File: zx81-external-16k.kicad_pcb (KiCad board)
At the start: 2 copper layers, 59.5 x 39 mm, 10 parts, among them J1 Connector ZX81, U1 CY62256-70PC, U2 74LS00

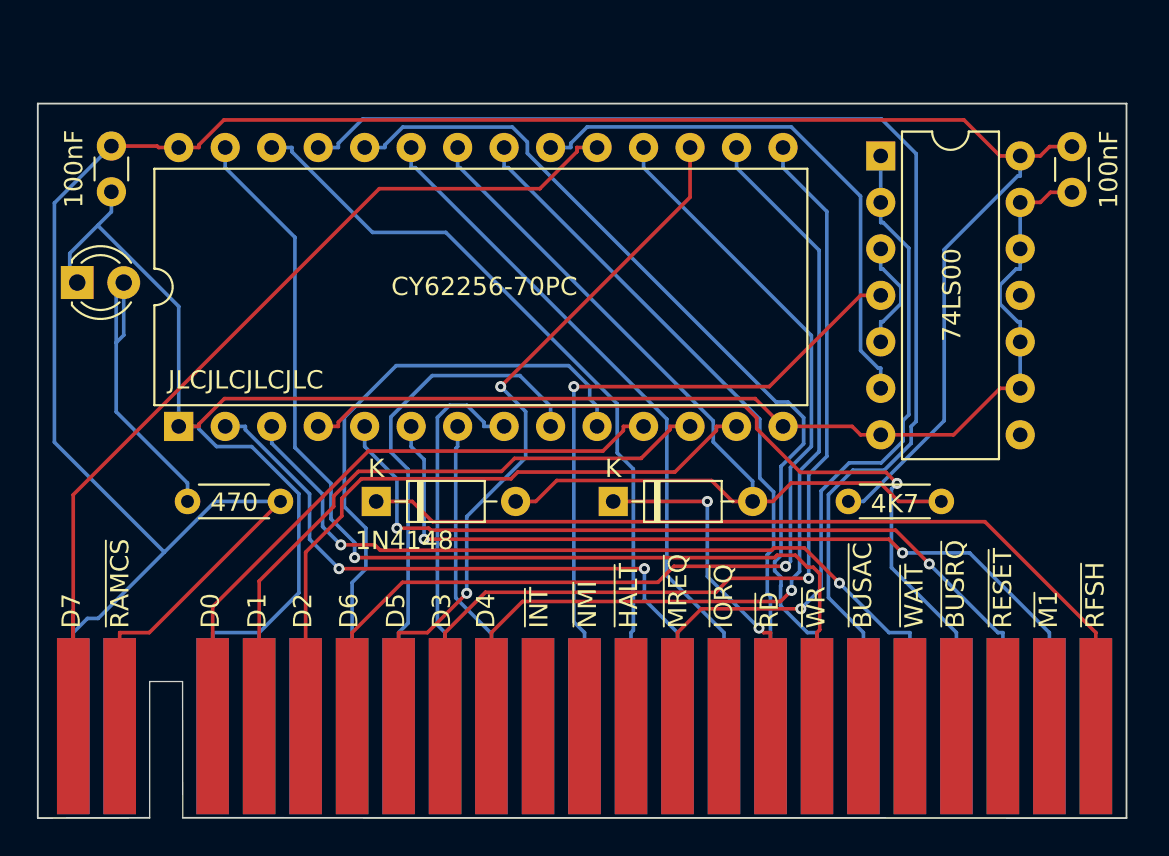
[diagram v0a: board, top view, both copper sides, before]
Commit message: v1.1
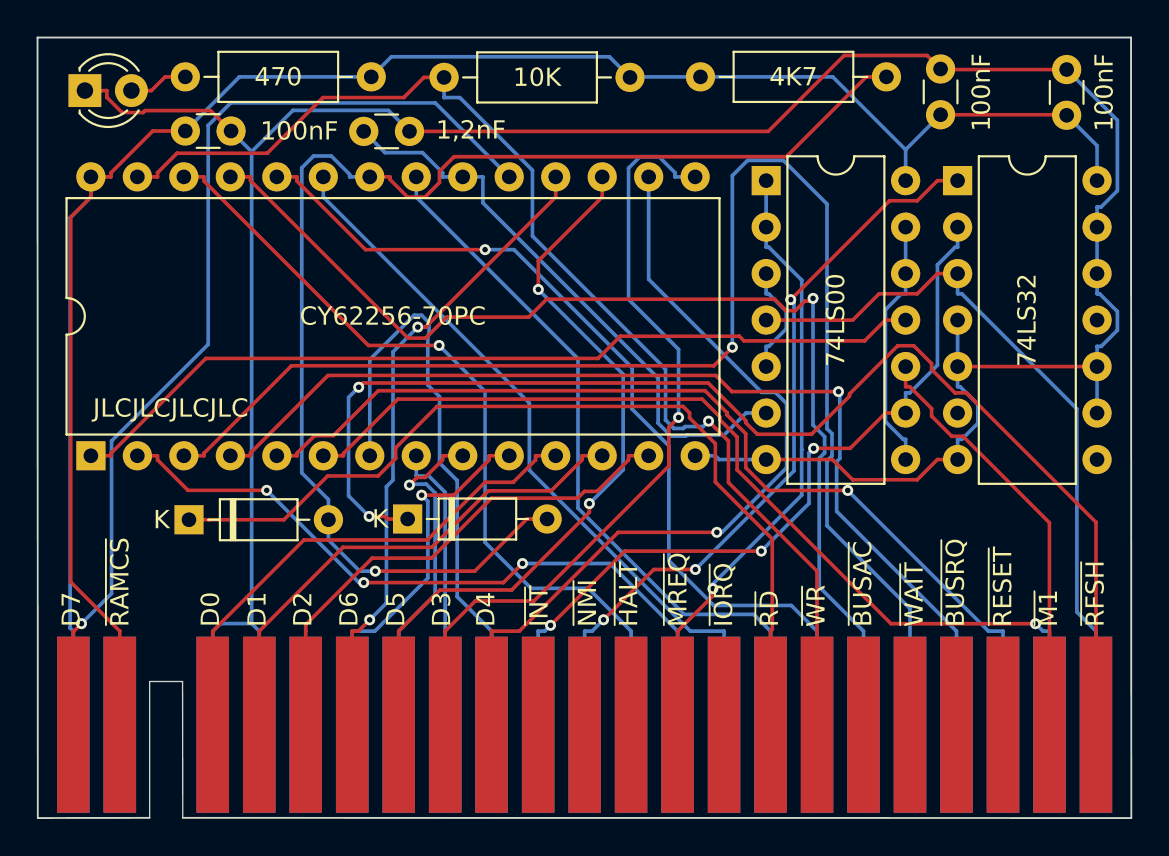
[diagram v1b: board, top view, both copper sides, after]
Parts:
- added C3: 100nF, Capacitor_THT:C_Disc_D3.0mm_W1.6mm_P2.50mm, F.Cu at (156.3, 90.1)
- added C4: 1,2nF, Capacitor_THT:C_Disc_D3.0mm_W1.6mm_P2.50mm, F.Cu at (117.8, 91.0)
- added R3: 10K, Resistor_THT:R_Axial_DIN0207_L6.3mm_D2.5mm_P10.16mm_Horizontal, F.Cu at (132.4, 88.0)
- added U3: 74LS32, Package_DIP:DIP-14_W7.62mm, F.Cu at (150.3, 93.7)
- R1, R2: footprint Resistor_THT:R_Axial_DIN0204_L3.6mm_D1.6mm_P5.08mm_Horizontal -> Resistor_THT:R_Axial_DIN0207_L6.3mm_D2.5mm_P10.16mm_Horizontal
- moved R2 24.6 mm to (136.2, 88.0)
- moved R1 23.7 mm to (118.3, 88.0)
- moved D3 23.2 mm to (108.3, 112.2)
- moved D1 10.5 mm to (102.6, 88.8)
- moved C2 7.39 mm to (149.4, 90.1), turned to 90 degrees
- moved U2 6.40 mm to (139.8, 93.7)
- moved U1 5.06 mm to (102.9, 108.7)
- moved C1 4.12 mm to (108.1, 91.0), turned to 0 degrees
- moved D2 1.97 mm to (120.2, 112.2)
- moved J1 0.08 mm to (131.2, 124.4)
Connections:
- J1 pad A13: unconnected-(J1-A15-PadA13) -> A15
- J1 pad A14: Net-(J1-PadA14) -> A14
- J1 pad A25: unconnected-(J1-~{ROMCS}-PadA25) -> Net-(J1-~{ROMCS})
- J1 pad B24: unconnected-(J1-~{M1}-PadB24) -> ~{M1}
- U1 pad 1: GND -> Net-(U1-A14)
- U2 pad 10: GND -> ~{M1}
- U2 pad 11: unconnected-(U2-Pad11) -> Net-(U1-A14)
- U2 pad 12: GND -> Net-(U2-Pad12)
- U2 pad 13: GND -> Net-(U2-Pad12)
- U2 pad 4: Net-(J1-PadA14) -> Net-(J1-~{ROMCS})
- U2 pad 8: unconnected-(U2-Pad8) -> Net-(U2-Pad12)
- U2 pad 9: GND -> A15
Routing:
- net Net-(U1-A14): track 0.00 -> 47.9 mm
- net A15: track 0.00 -> 43.3 mm, vias 0 -> 3
- net A14: track 0.00 -> 41.4 mm, vias 0 -> 3
- net Net-(J1-PadA14): track 40.2 -> 0.00 mm, vias 1 -> 0
- net Net-(J1-~{ROMCS}): track 0.00 -> 39.4 mm
- net GND: track 116.3 -> 151.0 mm
- net A7: track 48.9 -> 78.9 mm, vias 2 -> 1
- net Net-(D3-K): track 21.6 -> 49.4 mm, vias 2 -> 0
- net D6: track 60.1 -> 35.0 mm, vias 1 -> 2
- net ~{M1}: track 0.00 -> 23.3 mm
- net Net-(D2-A): track 51.1 -> 71.2 mm, vias 0 -> 1
- net Net-(D2-K): track 50.0 -> 68.8 mm, vias 0 -> 2
- net A0: track 39.0 -> 20.9 mm, vias 0 -> 1
- net +5V: track 144.9 -> 127.0 mm
- net Net-(D1-A): track 17.4 -> 3.26 mm
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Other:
- board size 59.5 x 39 mm -> 59.8 x 42.7 mm
- board text added: "ZX81 16/32K RAM v1.1 - by ZXINFO"
- board text removed: "ZX81 External 16k WRX RAM v1.0 - by ZXINFO"
